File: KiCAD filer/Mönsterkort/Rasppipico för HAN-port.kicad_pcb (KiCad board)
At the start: 2 copper layers, 33.8 x 78 mm, 3 parts, among them J1 RJ12

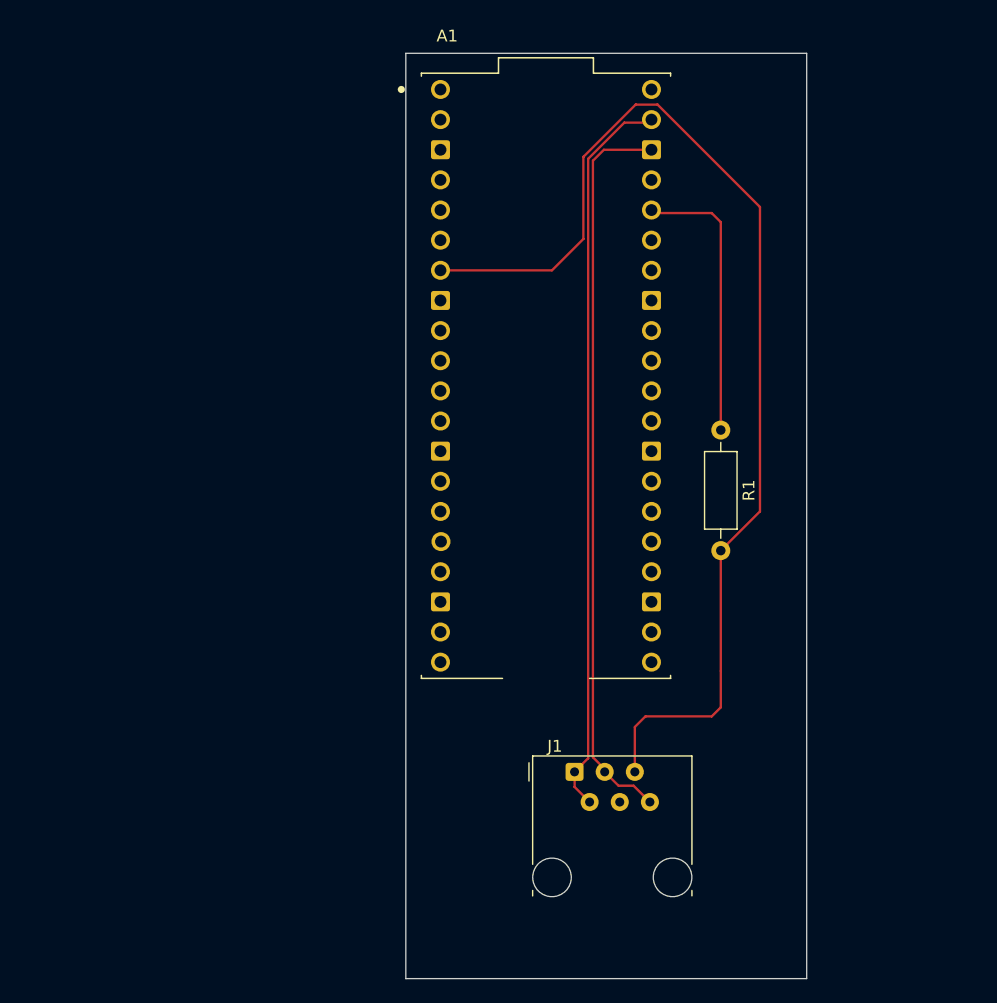
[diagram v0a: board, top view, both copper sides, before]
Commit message: Uppdatering av filer och la till stl filer
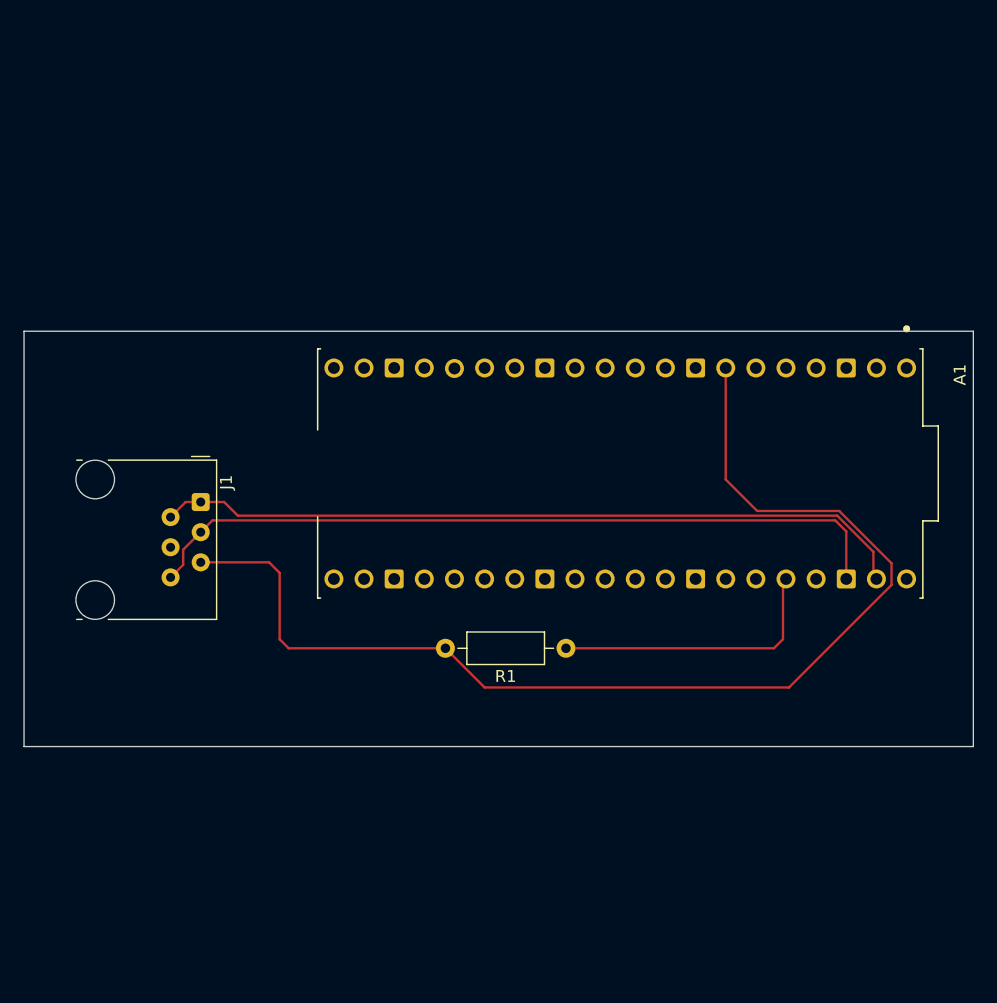
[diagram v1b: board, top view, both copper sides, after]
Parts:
- moved J1 38.9 mm to (112.9, 90.4), turned to -90 degrees
- moved R1 22.5 mm to (143.7, 102.7), turned to 180 degrees
- moved A1 10.3 mm to (148.2, 88.0), turned to -90 degrees
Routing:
- net /Data out: track 95.6 -> 97.6 mm
- net VCC: track 61.6 -> 63.5 mm
- net GND: track 62.4 -> 64.1 mm
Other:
- board size 33.8 x 78 mm -> 80 x 35 mm
